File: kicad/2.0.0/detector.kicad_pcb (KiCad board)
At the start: 4 copper layers, 33 x 29.3 mm, 45 parts, among them J1 Conn_01x05_Male, J2 Conn_01x05_Male, U1 LT1761-5, U2 LT1964-5, U3 REF5010ID, U4 OPA2197xD, U5 OPA2197xD

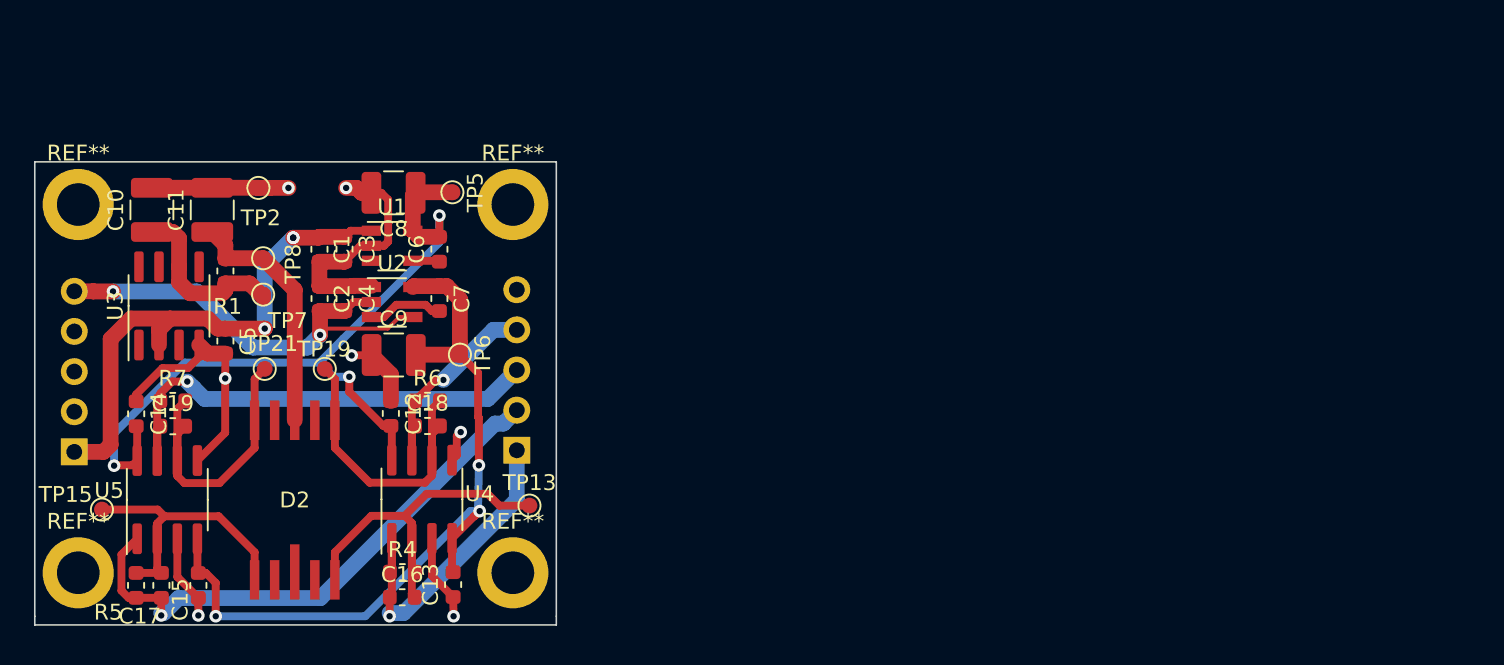
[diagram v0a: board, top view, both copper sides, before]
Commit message: reworked detector 2.0.0 pcb
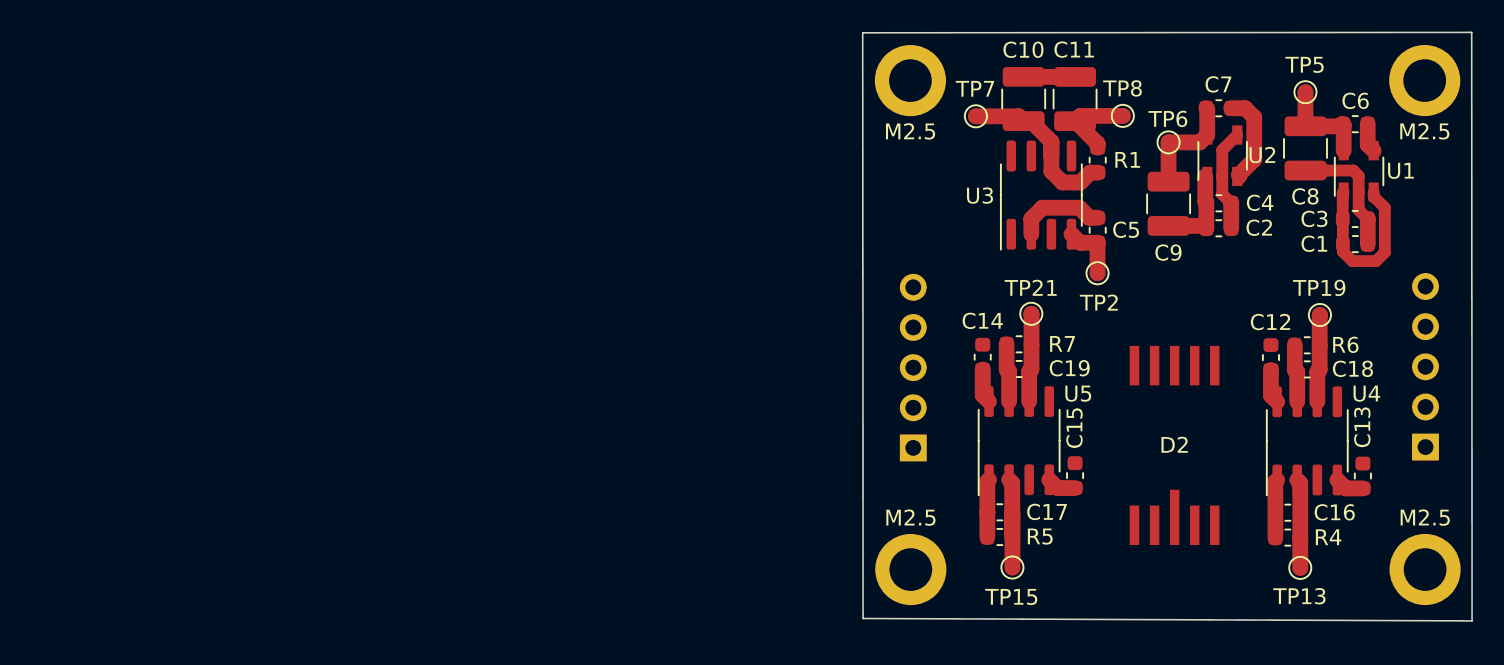
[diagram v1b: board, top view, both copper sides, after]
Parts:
- removed REF** (x2): MountingHole_2.7mm_M2.5_ISO7380_Pad, MountingHole:MountingHole_2.7mm_M2.5_ISO7380_Pad
- added M2.5: MountingHole_2.7mm_M2.5_ISO7380_Pad, MountingHole:MountingHole_2.7mm_M2.5_ISO7380_Pad, F.Cu at (180.7, 116.4)
- added M2.5: MountingHole_2.7mm_M2.5_ISO7380_Pad, MountingHole:MountingHole_2.7mm_M2.5_ISO7380_Pad, F.Cu at (148.2, 116.4)
- moved C1 65.5 mm to (176.3, 126.7), turned to 0 degrees
- moved C3 64.0 mm to (176.3, 125.1), turned to 0 degrees
- moved TP19 63.1 mm to (174.1, 131.2)
- moved U1 61.3 mm to (176.5, 122.1), turned to 90 degrees
- moved C6 58.5 mm to (176.3, 119.1), turned to 180 degrees
- moved C13 58.0 mm to (176.8, 141.4), turned to 270 degrees
- moved C8 57.8 mm to (173.2, 120.7), turned to 270 degrees
- moved TP15 57.7 mm to (154.6, 147.2)
- moved M2.5 57.7 mm to (180.7, 147.3)
- moved J2 57.5 mm to (180.7, 139.5)
- moved C2 57.1 mm to (167.7, 125.7), turned to 0 degrees
- moved C16 56.3 mm to (172.0, 143.7)
- moved U4 56.1 mm to (173.3, 139.2)
- moved R4 56.1 mm to (172.0, 145.3)
- moved C15 55.9 mm to (158.6, 141.4), turned to 270 degrees
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- renumbered REF** to M2.5
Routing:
- net -5V: track 50.0 -> 10.5 mm, vias 3 -> 0
- net +5V: track 50.0 -> 10.6 mm, vias 3 -> 0
- net GND: track 57.6 -> 20.9 mm, vias 7 -> 0
- net /-Y1: track 35.4 -> 3.67 mm, vias 1 -> 0
- net /-X2: track 30.7 -> 3.69 mm, vias 1 -> 0
- net -12V: track 28.7 -> 6.53 mm, vias 2 -> 0
- net Net-(C16-Pad2): track 23.5 -> 5.64 mm
- net /-X1: track 21.3 -> 3.69 mm, vias 1 -> 0
- net +12V: track 33.3 -> 16.8 mm, vias 3 -> 0
- net Net-(C18-Pad2): track 19.8 -> 5.56 mm
- net Net-(C19-Pad2): track 18.6 -> 5.62 mm
- net Net-(C17-Pad2): track 18.0 -> 7.20 mm
- net /-Y2: track 14.4 -> 3.64 mm, vias 1 -> 0
- net Net-(C11-Pad1): track 15.5 -> 5.43 mm
- net Net-(C7-Pad2): track 4.78 -> 5.85 mm
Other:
- board size 33 x 29.3 mm -> 38.6 x 37.2 mm
